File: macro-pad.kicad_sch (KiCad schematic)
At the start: 0 parts

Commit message: keyboard matrix and microcontroller sch
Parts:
- added A2: RaspberryPi_Pico_W, Module:RaspberryPi_Pico_W_SMD_HandSolder, symbol MCU_Module:RaspberryPi_Pico_W
- added D1, D2, D3, D4, D5, D6, D7, D8, D9: 1N4148, Diode_THT:D_DO-35_SOD27_P7.62mm_Horizontal, symbol Diode:1N4148
- added SW1, SW2, SW3, SW4, SW5, SW6, SW7, SW8, SW9: SW_Push_45deg, symbol Switch:SW_Push_45deg
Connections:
- new net: D9.2 (A), SW9.2
- new net: D5.2 (A), SW5.2
- new net: D1.2 (A), SW1.2
- new net: D2.2 (A), SW2.2
- new net: A2.13 (GND), A2.18 (GND), A2.23 (GND), A2.28 (GND), A2.3 (GND), A2.38 (GND), A2.8 (GND)
- new net: D6.2 (A), SW6.2
- new net: D7.2 (A), SW7.2
- new net: D3.2 (A), SW3.2
- new net: D4.2 (A), SW4.2
- new net: D8.2 (A), SW8.2
- new net col0: SW1.1, SW4.1, SW7.1
- new net col1: SW2.1, SW5.1, SW8.1
- new net col2: SW3.1, SW6.1, SW9.1
- new net row0: D1.1 (K), D2.1 (K), D3.1 (K)
- new net row1: D4.1 (K), D5.1 (K), D6.1 (K)
- new net row2: D7.1 (K), D8.1 (K), D9.1 (K)

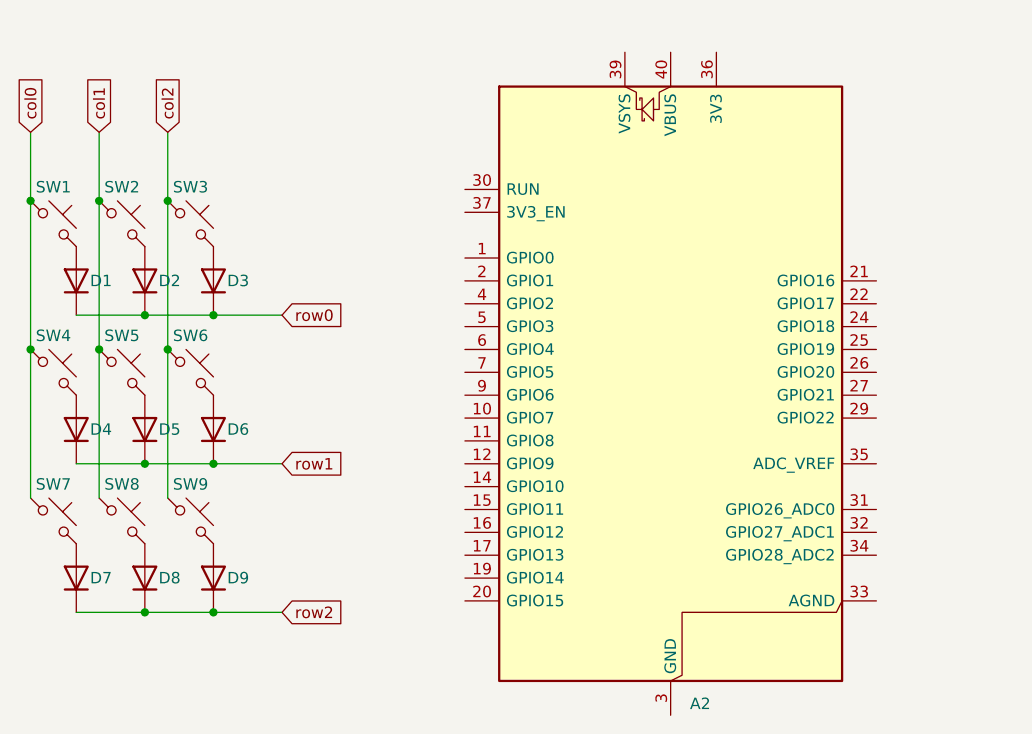
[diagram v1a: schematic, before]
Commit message: finished sch, inprogress pcb
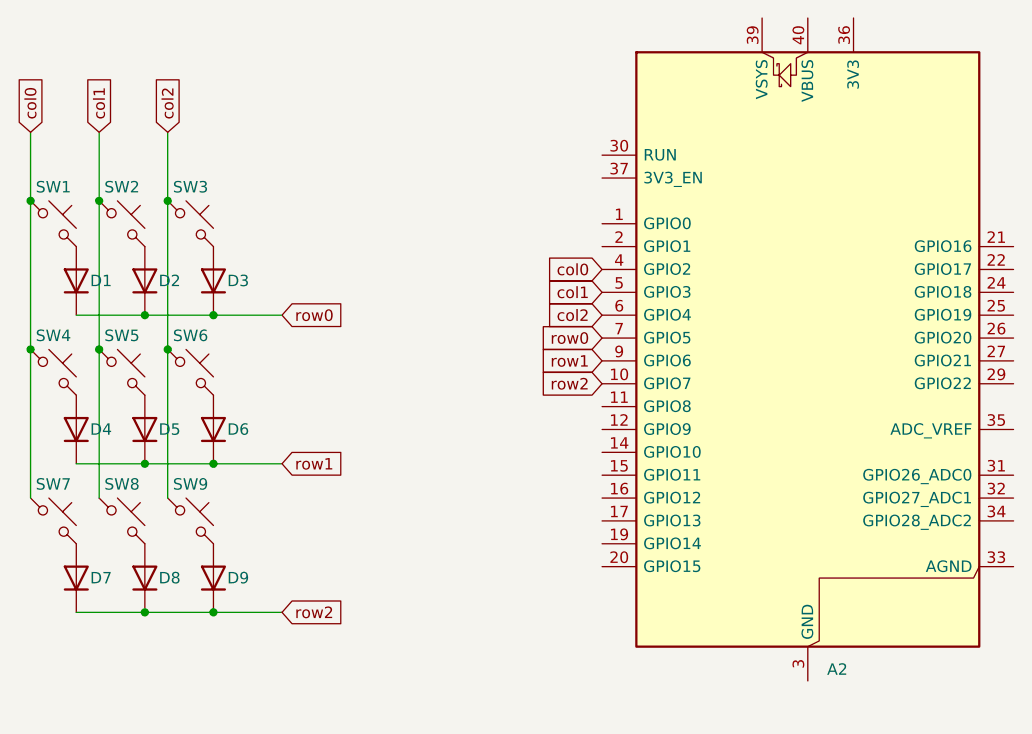
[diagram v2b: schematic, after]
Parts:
- SW1, SW2, SW3, SW4, SW5, SW6, SW7, SW8, SW9: footprint (none) -> Button_Switch_Keyboard:SW_Cherry_MX_1.00u_PCB
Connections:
- net col0: now also A2.4 (GPIO2)
- net col1: now also A2.5 (GPIO3)
- net col2: now also A2.6 (GPIO4)
- net row0: now also A2.7 (GPIO5)
- net row1: now also A2.9 (GPIO6)
- net row2: now also A2.10 (GPIO7)
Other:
- moved on the sheet: A2
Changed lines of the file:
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@@
+		)
+	)
+	(global_label "row2"
+		(shape input)
+		(at 154.94 114.3 180)
+		(fields_autoplaced yes)
+		(effects
+			(font
+				(size 1.27 1.27)
+			)
+			(justify right)
+		)
+		(property "Intersheetrefs" "${INTERSHEET_REFS}"
+			(at 147.4796 114.3 0)
+			(effects
+				(font
+					(size 1.27 1.27)
+				)
+				(justify right)
+				(hide yes)
+			)
 		)
 	)
@@
 		)
 	)
+	(global_label "row1"
+		(shape input)
+		(at 154.94 111.76 180)
+		(fields_autoplaced yes)
+		(effects
+			(font
+				(size 1.27 1.27)
+			)
+			(justify right)
+		)
+		(property "Intersheetrefs" "${INTERSHEET_REFS}"
+			(at 147.4796 111.76 0)
+			(effects
+				(font
+					(size 1.27 1.27)
+				)
+				(justify right)
+				(hide yes)
+			)
+		)
+	)
 	(global_label "row0"
 		(shape input)
@@
 	(global_label "col0"
 		(shape input)
+		(at 154.94 101.6 180)
+		(fields_autoplaced yes)
+		(effects
+			(font
+				(size 1.27 1.27)
+			)
+			(justify right)
+		)
+		(property "Intersheetrefs" "${INTERSHEET_REFS}"
+			(at 147.8425 101.6 0)
+			(effects
+				(font
+					(size 1.27 1.27)
+				)
+				(justify right)
+				(hide yes)
+			)
+		)
+	)
+	(global_label "col1"
+		(shape input)
+		(at 154.94 104.14 180)
+		(fields_autoplaced yes)
+		(effects
+			(font
+				(size 1.27 1.27)
+			)
+			(justify right)
+		)
+		(property "Intersheetrefs" "${INTERSHEET_REFS}"
+			(at 147.8425 104.14 0)
+			(effects
+				(font
+					(size 1.27 1.27)
+				)
+				(justify right)
+				(hide yes)
+			)
+		)
+	)
+	(global_label "col2"
+		(shape input)
+		(at 154.94 106.68 180)
+		(fields_autoplaced yes)
+		(effects
+			(font
+				(size 1.27 1.27)
+			)
+			(justify right)
+		)
+		(property "Intersheetrefs" "${INTERSHEET_REFS}"
+			(at 147.8425 106.68 0)
+			(effects
+				(font
+					(size 1.27 1.27)
+				)
+				(justify right)
+				(hide yes)
+			)
+		)
+	)
+	(global_label "row0"
+		(shape input)
+		(at 154.94 109.22 180)
+		(fields_autoplaced yes)
+		(effects
+			(font
+				(size 1.27 1.27)
+			)
+			(justify right)
+		)
+		(property "Intersheetrefs" "${INTERSHEET_REFS}"
+			(at 147.4796 109.22 0)
+			(effects
+				(font
+					(size 1.27 1.27)
+				)
+				(justify right)
+				(hide yes)
+			)
+		)
+	)
+	(global_label "col0"
+		(shape input)
 		(at 91.44 86.36 90)
 		(fields_autoplaced yes)
@@
 			)
 		)
-		(property "Footprint" ""
+		(property "Footprint" "Button_Switch_Keyboard:SW_Cherry_MX_1.00u_PCB"
 			(at 109.22 129.54 0)
 			(effects
@@
 	(symbol
 		(lib_id "MCU_Module:RaspberryPi_Pico_W")
-		(at 162.56 115.57 0)
+		(at 177.8 111.76 0)
 		(unit 1)
 		(exclude_from_sim no)
@@
 		(fields_autoplaced yes)
 		(property "Reference" "A2"
-			(at 164.7033 149.86 0)
+			(at 179.9433 146.05 0)
 			(effects
 				(font
@@
 		)
 		(property "Value" "RaspberryPi_Pico_W"
-			(at 164.7033 152.4 0)
+			(at 179.9433 148.59 0)
 			(effects
 				(font
@@
 		)
 		(property "Footprint" "Module:RaspberryPi_Pico_W_SMD_HandSolder"
-			(at 162.56 162.56 0)
+			(at 177.8 158.75 0)
 			(effects
 				(font
@@
 		)
 		(property "Datasheet" "https://datasheets.raspberrypi.com/picow/pico-w-datasheet.pdf"
-			(at 162.56 165.1 0)
+			(at 177.8 161.29 0)
 			(effects
 				(font
@@
 		)
 		(property "Description" "Versatile and inexpensive wireless microcontroller module powered by RP2040 dual-core Arm Cortex-M0+ processor up to 133 MHz, 264kB SRAM, 2MB QSPI flash, Infineon CYW43439 2.4GHz 802.11n wireless LAN; also supports Raspberry Pi Pico 2 W"
-			(at 162.56 167.64 0)
+			(at 177.8 163.83 0)
 			(effects
 				(font
@@
 			)
 		)
-		(property "Footprint" ""
+		(property "Footprint" "Button_Switch_Keyboard:SW_Cherry_MX_1.00u_PCB"
 			(at 109.22 113.03 0)
 			(effects
@@
 			)
 		)
-		(property "Footprint" ""
+		(property "Footprint" "Button_Switch_Keyboard:SW_Cherry_MX_1.00u_PCB"
 			(at 93.98 129.54 0)
 			(effects
@@
 			)
 		)
-		(property "Footprint" ""
+		(property "Footprint" "Button_Switch_Keyboard:SW_Cherry_MX_1.00u_PCB"
 			(at 93.98 113.03 0)
 			(effects
@@
 			)
 		)
-		(property "Footprint" ""
+		(property "Footprint" "Button_Switch_Keyboard:SW_Cherry_MX_1.00u_PCB"
 			(at 93.98 96.52 0)
 			(effects
@@
 			)
 		)
-		(property "Footprint" ""
+		(property "Footprint" "Button_Switch_Keyboard:SW_Cherry_MX_1.00u_PCB"
 			(at 101.6 129.54 0)
 			(effects
@@
 			)
 		)
-		(property "Footprint" ""
+		(property "Footprint" "Button_Switch_Keyboard:SW_Cherry_MX_1.00u_PCB"
 			(at 101.6 113.03 0)
 			(effects
@@
 			)
 		)
-		(property "Footprint" ""
+		(property "Footprint" "Button_Switch_Keyboard:SW_Cherry_MX_1.00u_PCB"
 			(at 101.6 96.52 0)
 			(effects
@@
 			)
 		)
-		(property "Footprint" ""
+		(property "Footprint" "Button_Switch_Keyboard:SW_Cherry_MX_1.00u_PCB"
 			(at 109.22 96.52 0)
 			(effects
